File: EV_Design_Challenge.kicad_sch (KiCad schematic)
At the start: 15 parts, among them J1 WAGO-2604-1102, J2 WAGO-2604-1102, J5 WAGO-2604-1102

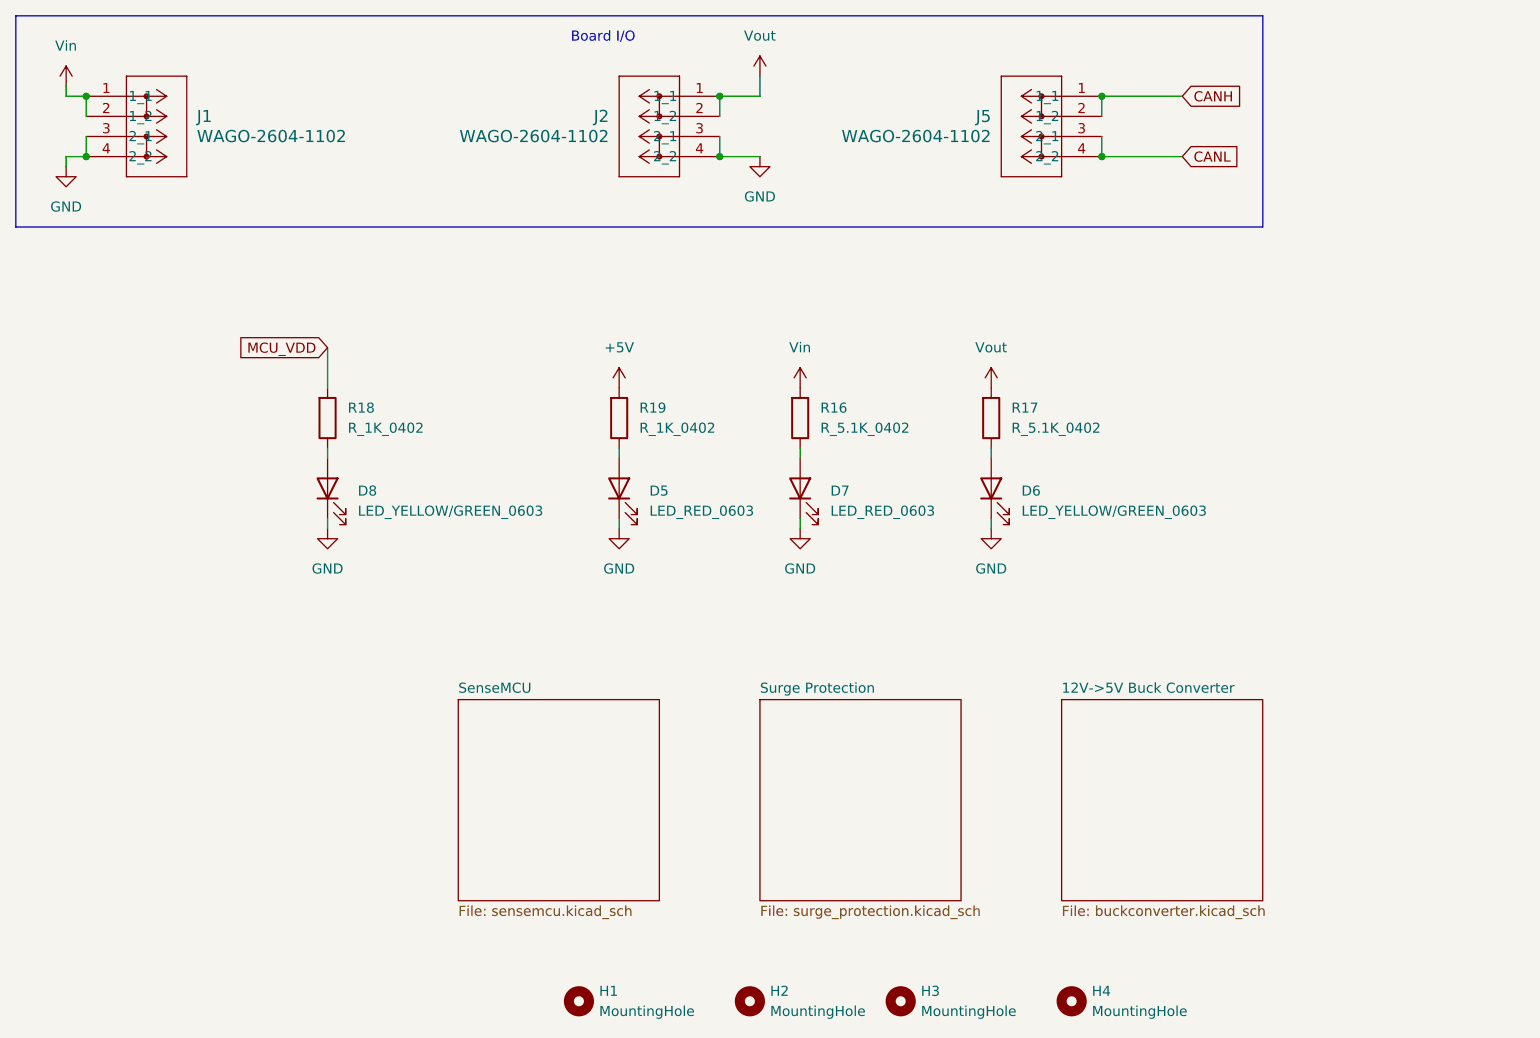
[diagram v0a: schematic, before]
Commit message: Add files via upload
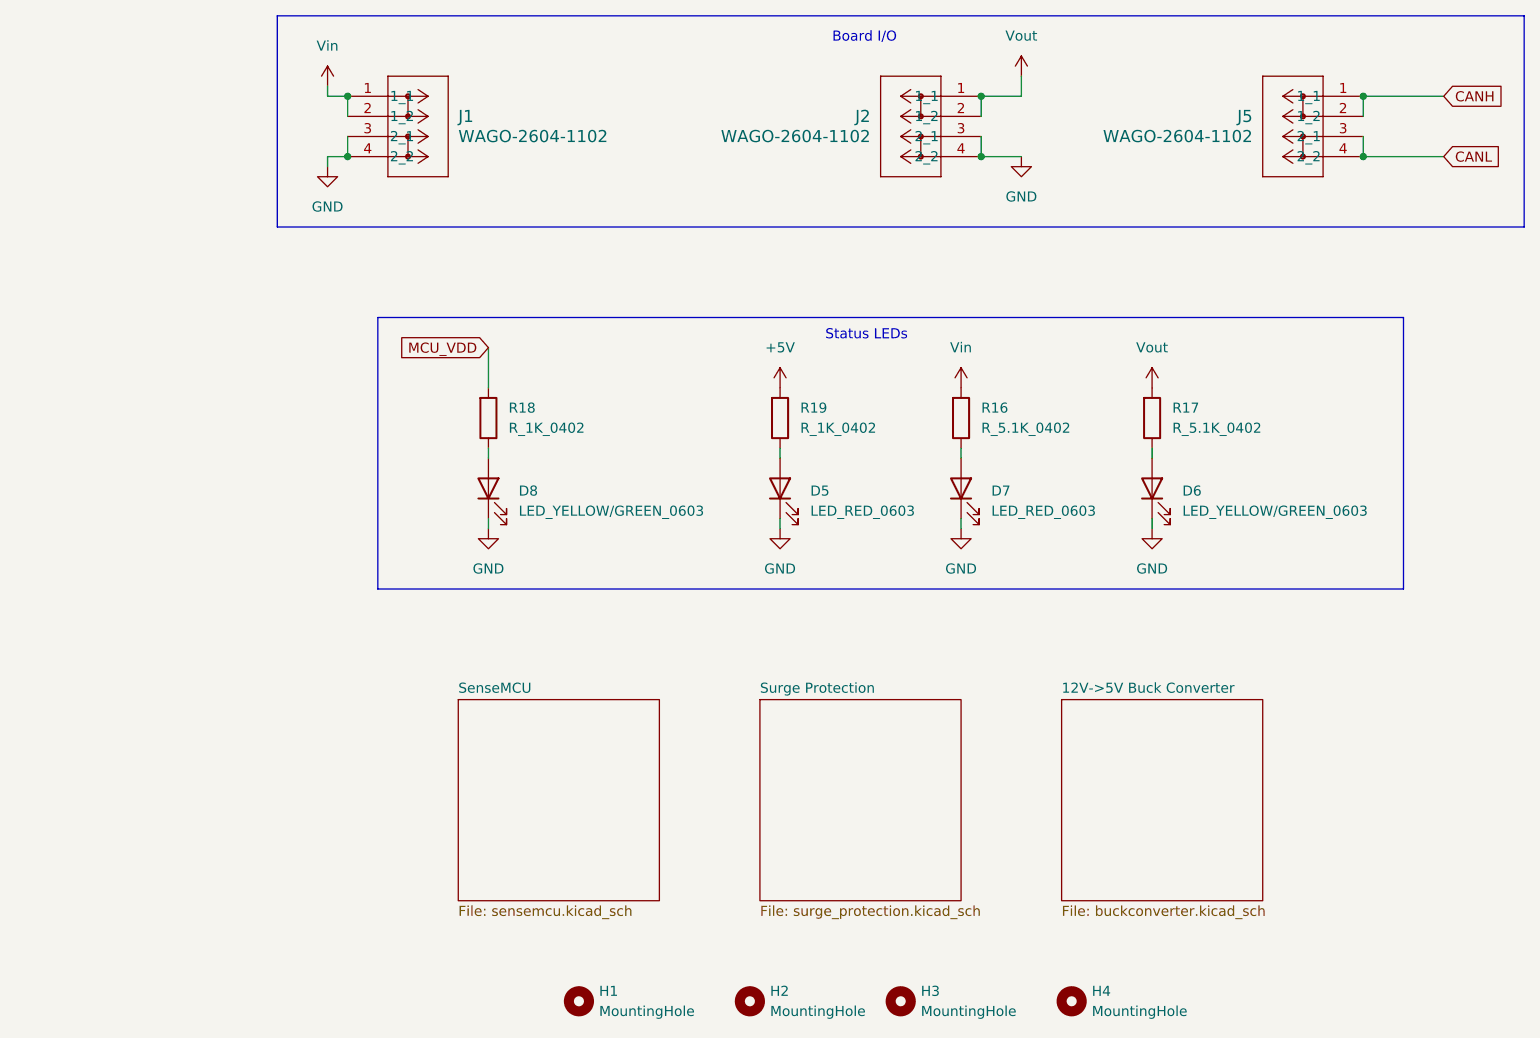
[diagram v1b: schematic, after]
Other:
- note added: "Status LEDs"
- moved on the sheet: D5, D6, D7, D8, J1, J2, J5, R16, R17, R18, R19
